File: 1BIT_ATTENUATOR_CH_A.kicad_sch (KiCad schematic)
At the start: 9 parts, among them IC901 ${DEVICE}, IC902 ${DEVICE}, IC903 ${DEVICE}

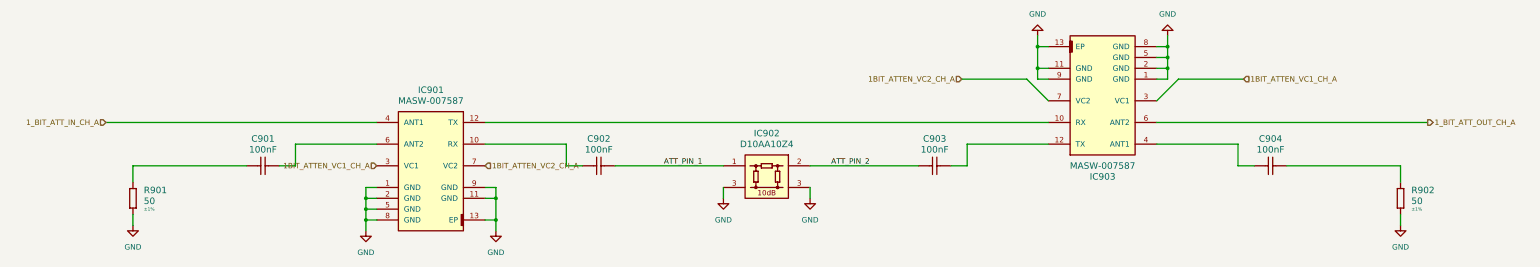
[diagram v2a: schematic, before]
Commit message: WIP snapshot
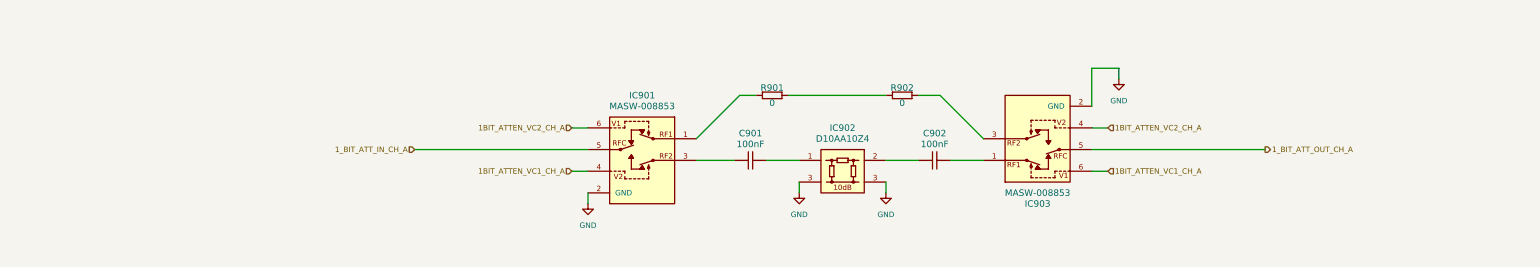
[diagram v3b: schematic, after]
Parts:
- removed C903, C904: 100nF, Capacitors SMD:CAPC1005X55N, symbol CERN:Capacitors SMD/CC0402_100NF_50V_10%_X7R
- removed IC901, IC903: ${DEVICE}, ICs And Semiconductors SMD:QFN50P300X300X100-13N-S125, symbol CERN:Analog & Interface/MASW-007587
- removed R901, R902: 50, Resistors SMD:RESC1608X55N, symbol CERN:Resistors SMD/R0603_50R_1%_0.1W_100PPM
- added IC901, IC903: ${DEVICE}, ICs And Semiconductors SMD:SOT65P210X110-6N, symbol CERN:Analog & Interface/MASW-008853
- added R901, R902: 0, Resistors SMD:RESC1005X40N, symbol CERN:Resistors SMD/R0402_0R_JUMPER
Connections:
- net ATT_PIN_2 is gone; now on an unnamed net: IC902.2 (OUT)
- net 1BIT_ATTEN_VC1_CH_A: now also IC901.4 (V2), IC903.6 (V1)
- net 1BIT_ATTEN_VC2_CH_A: now also IC901.6 (V1), IC903.4 (V2)
- net 1_BIT_ATT_IN_CH_A: now also IC901.5 (RFC)
- net 1_BIT_ATT_OUT_CH_A: now also IC903.5 (RFC)
- net GND: now also IC901.2 (GND), IC903.2 (GND)
- net at C901.1: now also IC901.3 (RF2)
- net at C901.2: now also IC902.1 (IN)
- net ATT_PIN_1: no longer names the net of C902.2
- net ATT_PIN_1: now also IC903.1 (RF1); no longer IC902.1 (IN)
- new net: R901.2, R902.1
- new net: IC903.3 (RF2), R902.2
- new net: IC901.1 (RF1), R901.1
